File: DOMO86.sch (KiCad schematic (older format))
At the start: 176 parts, among them SW1 Rotary_Encoder_Switch, U1 proton_c, U2 OLED-SSD1306

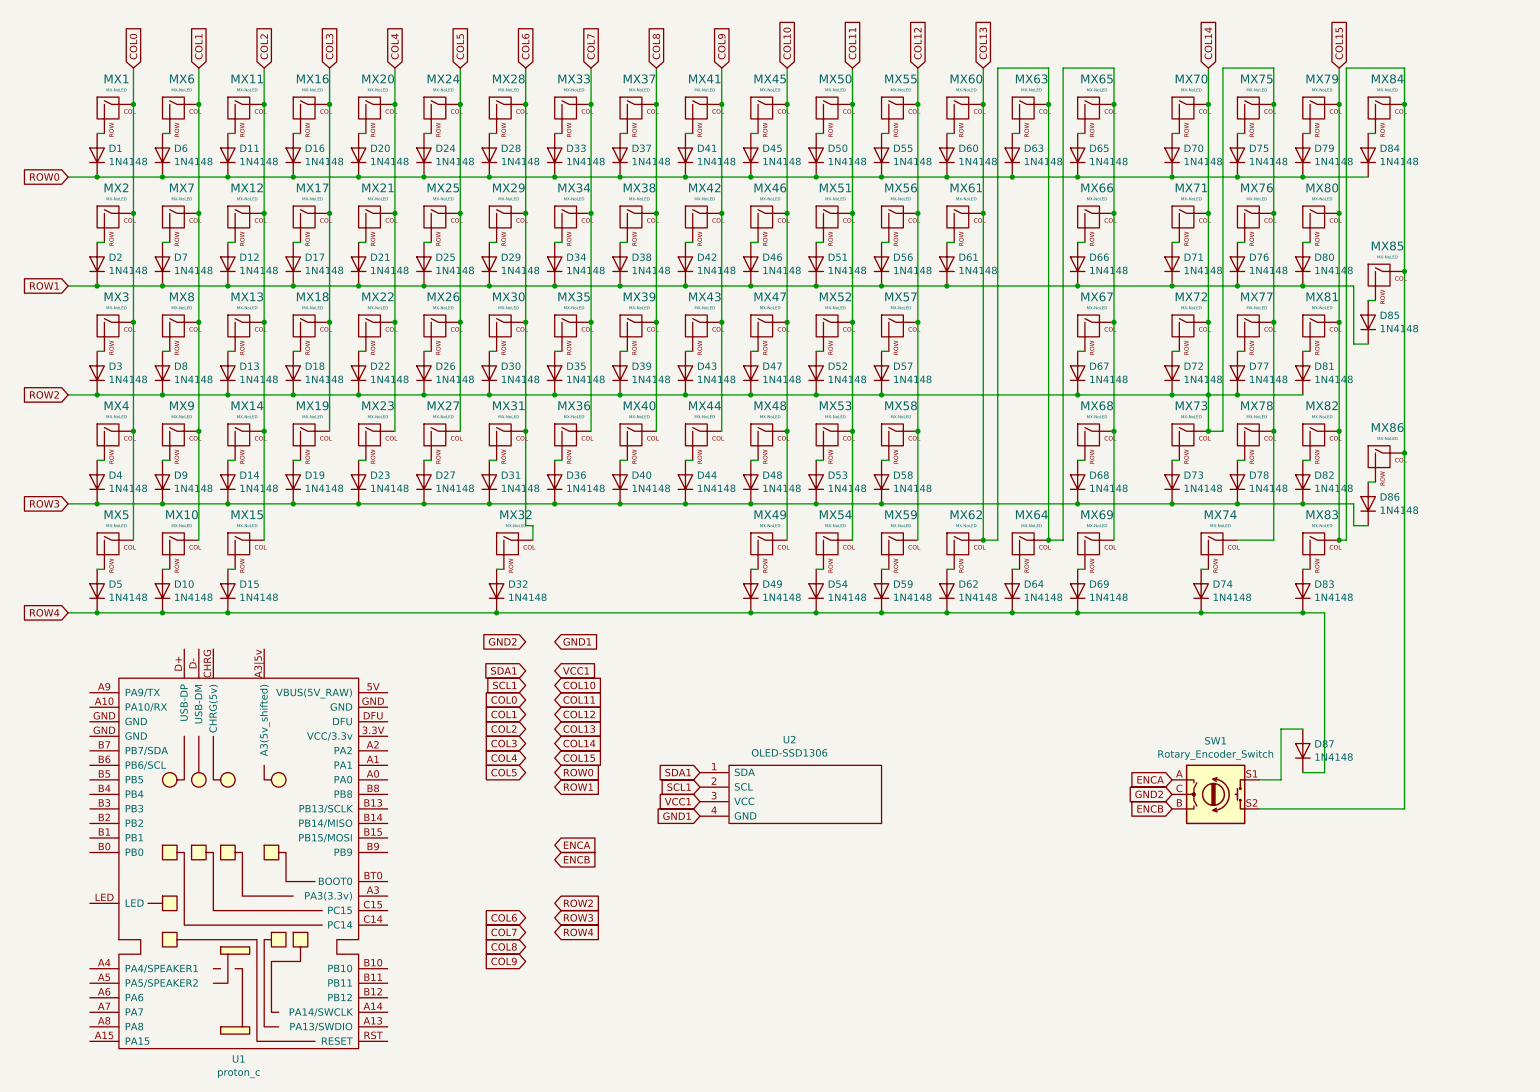
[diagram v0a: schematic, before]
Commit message: Finished routing
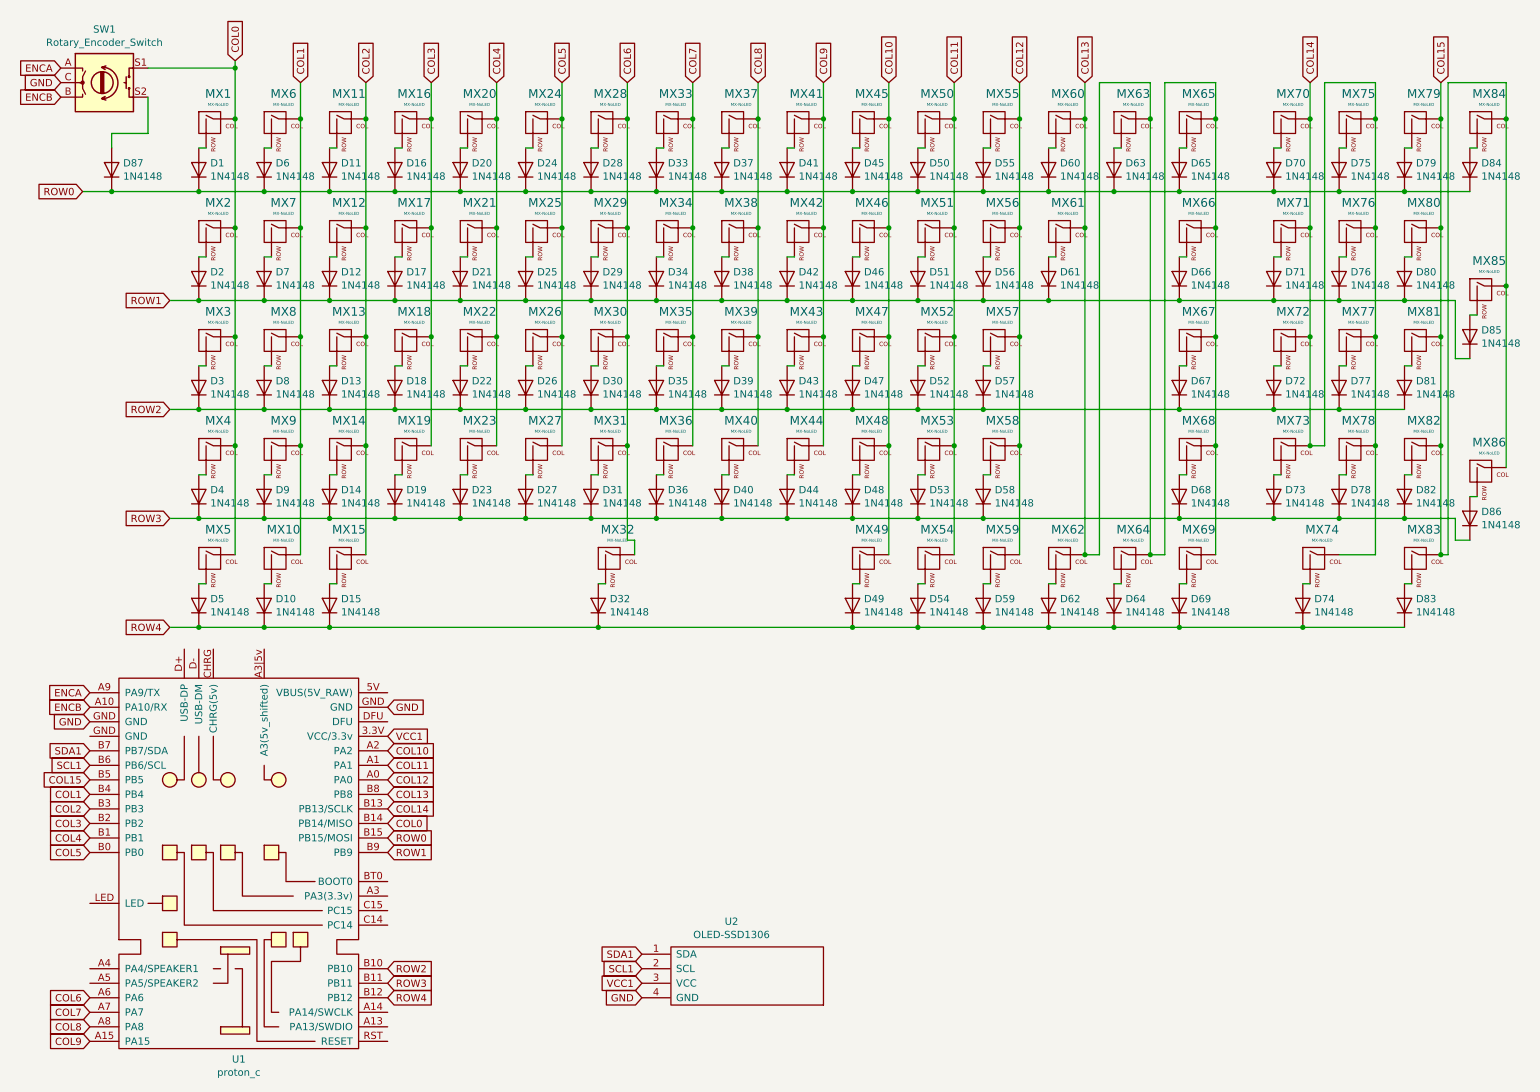
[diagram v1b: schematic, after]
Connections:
- net GND1 is gone; now on net GND: U2.4 (GND)
- net GND2 is gone; now on net GND: SW1.C
- net COL0: now also SW1.S1, U1.B14 (PB14/MISO)
- net COL1: now also U1.B4 (PB4)
- net COL10: now also U1.A2 (PA2)
- net COL11: now also U1.A1 (PA1)
- net COL12: now also U1.A0 (PA0)
- net COL13: now also U1.B8 (PB8)
- net COL14: now also U1.B13 (PB13/SCLK); no longer D13.1 (K), D18.1 (K), D22.1 (K), D26.1 (K), D3.1 (K), D30.1 (K), D35.1 (K), D39.1 (K), D43.1 (K), D47.1 (K), D52.1 (K), D57.1 (K), D67.1 (K), D72.1 (K), D77.1 (K), D8.1 (K), D81.1 (K)
- net COL15: now also U1.B5 (PB5); no longer SW1.S2
- net COL2: now also U1.B3 (PB3)
- net COL3: now also U1.B2 (PB2)
- net COL4: now also U1.B1 (PB1)
- net COL5: now also U1.B0 (PB0)
- net COL6: now also U1.A6 (PA6)
- net COL7: now also U1.A7 (PA7)
- net COL8: now also U1.A8 (PA8)
- net COL9: now also U1.A15 (PA15)
- net ENCA: now also U1.A9 (PA9/TX)
- net ENCB: now also U1.A10 (PA10/RX)
- net ROW0: now also D87.1 (K), U1.B15 (PB15/MOSI)
- net ROW1: now also U1.B9 (PB9)
- net ROW3: now also U1.B11 (PB11)
- net ROW4: now also U1.B12 (PB12); no longer D87.1 (K)
- net SCL1: now also U1.B6 (PB6/SCL)
- net SDA1: now also U1.B7 (PB7/SDA)
- net VCC1: now also U1.3.3V (VCC/3.3v)
- net ROW2: now reaches U1.B10 (PB10)
- net ROW2: now also D13.1 (K), D18.1 (K), D22.1 (K), D26.1 (K), D3.1 (K), D30.1 (K), D35.1 (K), D39.1 (K), D43.1 (K), D47.1 (K), D52.1 (K), D57.1 (K), D67.1 (K), D72.1 (K), D77.1 (K), D8.1 (K), D81.1 (K)
- net GND: now reaches U1.GND
- net at D87.2 (A): now also SW1.S2; no longer SW1.S1
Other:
- moved on the sheet: D1, D10, D11, D12, D13, D14, D15, D16, D17, D18, D19, D2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
